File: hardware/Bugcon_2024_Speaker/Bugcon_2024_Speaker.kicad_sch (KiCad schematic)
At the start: 53 parts, among them J1 OLED, J2 Add_On, J4 Battery, J5 Battery, P1 USB_C_Plug_USB2.0, Q1 DMG3415U-7, SW1 ON, U1 ESP32-C6-WROOM-1U-N4, U2 XC6220B331MR-G

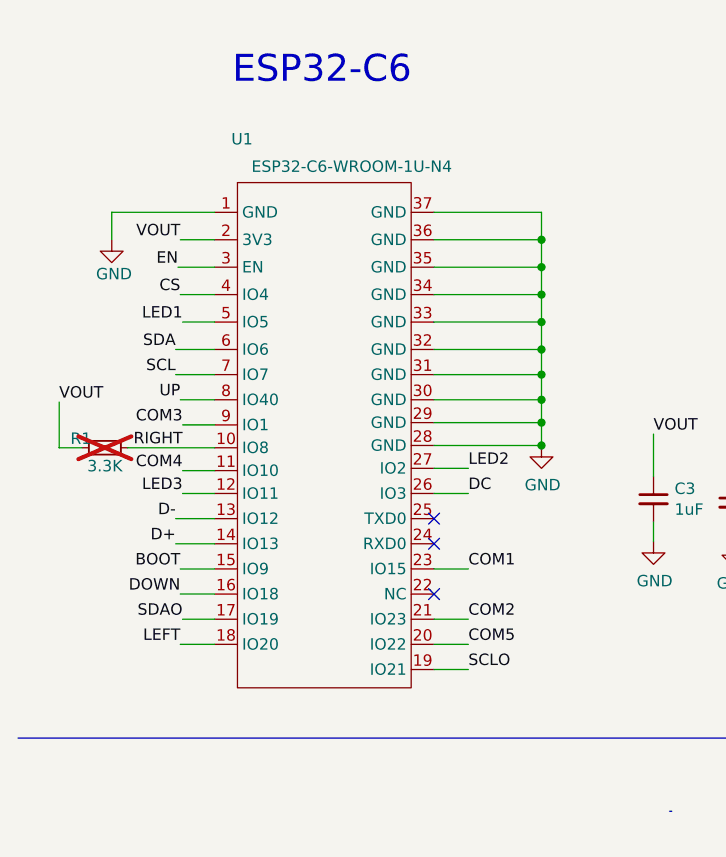
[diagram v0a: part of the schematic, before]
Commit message: feat(Hw):Update_Labels_And_route
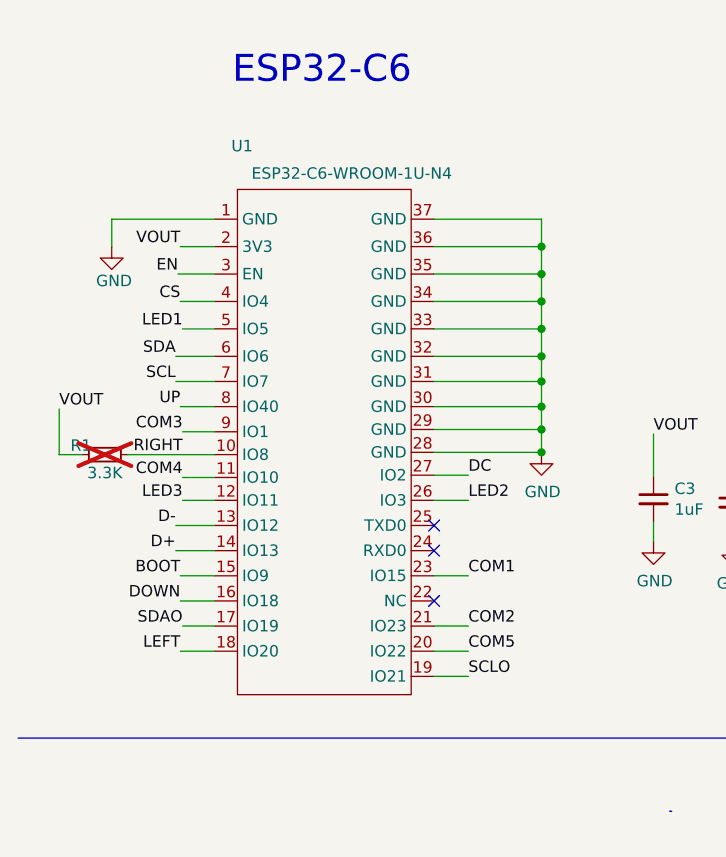
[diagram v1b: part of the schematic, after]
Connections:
- net DC: now also U1.27 (IO2); no longer U1.26 (IO3)
- net LED2: now also U1.26 (IO3); no longer U1.27 (IO2)
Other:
- moved on the sheet: R1, U1

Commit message: feat(Hw):Update_BOM
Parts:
- C1, C11, C12, C13, C14, C2, C3, C4, C5, C6, C7, D1, F1, J2, J4, J5, P1, Q1, R1, R2, R3, R4, R6, SW1, SW2, SW3, SW4, SW5, SW6, SW7, U2: Proveedor JLCPCB -> (none)
- D2, D3, D4, D5, D8: Proveedor (none) -> MOUSER
- J1: Proveedor (none) -> UNIT; manf# (none) -> GC9A01 Pantalla TFT LCD Circular 1.28 Pulgadas
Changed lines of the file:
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@@
 			)
 		)
-		(property "Proveedor" "JLCPCB"
+		(property "Proveedor" ""
 			(at 192.151 68.326 0)
 			(effects
@@
 			)
 		)
-		(property "Proveedor" "JLCPCB"
+		(property "Proveedor" ""
 			(at 193.294 55.118 0)
 			(effects
@@
 			)
 		)
-		(property "Proveedor" "JLCPCB"
+		(property "Proveedor" ""
 			(at 259.08 64.516 0)
 			(effects
@@
 			)
 		)
-		(property "Proveedor" "JLCPCB"
+		(property "Proveedor" ""
 			(at 193.294 52.578 0)
 			(effects
@@
 			)
 		)
-		(property "Proveedor" "JLCPCB"
+		(property "Proveedor" ""
 			(at 150.622 47.498 0)
 			(effects
@@
 			)
 		)
+		(property "Proveedor" "MOUSER"
+			(at 207.01 123.19 0)
+			(effects
+				(font
+					(size 1.27 1.27)
+				)
+				(hide yes)
+			)
+		)
 		(pin "3"
 		)
@@
 			)
 		)
-		(property "Proveedor" "JLCPCB"
+		(property "Proveedor" ""
 			(at 151.892 42.418 0)
 			(effects
@@
 			)
 		)
+		(property "Proveedor" "MOUSER"
+			(at 265.43 133.35 0)
+			(effects
+				(font
+					(size 1.27 1.27)
+				)
+				(hide yes)
+			)
+		)
 		(pin "3"
 		)
@@
 			)
 		)
-		(property "Proveedor" "JLCPCB"
+		(property "Proveedor" ""
 			(at 41.783 179.451 0)
 			(effects
@@
 			)
 		)
+		(property "Proveedor" "MOUSER"
+			(at 265.43 109.22 0)
+			(effects
+				(font
+					(size 1.27 1.27)
+				)
+				(hide yes)
+			)
+		)
 		(pin "3"
 		)
@@
 			)
 		)
-		(property "Proveedor" "JLCPCB"
+		(property "Proveedor" ""
 			(at 82.804 66.167 0)
 			(effects
@@
 			)
 		)
-		(property "Proveedor" "JLCPCB"
+		(property "Proveedor" ""
 			(at 259.08 48.006 0)
 			(effects
@@
 			)
 		)
-		(property "Proveedor" "JLCPCB"
+		(property "Proveedor" ""
 			(at 64.77 121.92 0)
 			(effects
@@
 			)
 		)
+		(property "Proveedor" "UNIT"
+			(at 143.51 121.92 0)
+			(effects
+				(font
+					(size 1.27 1.27)
+				)
+				(hide yes)
+			)
+		)
+		(property "manf#" "GC9A01 Pantalla TFT LCD Circular 1.28 Pulgadas"
+			(at 143.51 121.92 0)
+			(effects
+				(font
+					(size 1.27 1.27)
+				)
+				(hide yes)
+			)
+		)
 		(pin "3"
 		)
@@
 			)
 		)
-		(property "Proveedor" "JLCPCB"
+		(property "Proveedor" ""
 			(at 91.694 66.548 0)
 			(effects
@@
 			)
 		)
-		(property "Proveedor" "JLCPCB"
+		(property "Proveedor" ""
 			(at 146.304 180.848 0)
 			(effects
@@
 			)
 		)
-		(property "Proveedor" "JLCPCB"
+		(property "Proveedor" ""
 			(at 258.826 44.45 0)
 			(effects
@@
 			)
 		)
-		(property "Proveedor" "JLCPCB"
+		(property "Proveedor" ""
 			(at 100.584 66.548 0)
 			(effects
@@
 			)
 		)
-		(property "Proveedor" "JLCPCB"
+		(property "Proveedor" ""
 			(at 258.826 24.13 0)
 			(effects
@@
 			)
 		)
-		(property "Proveedor" "JLCPCB"
+		(property "Proveedor" ""
 			(at 131.064 57.658 0)
 			(effects
@@
 			)
 		)
-		(property "Proveedor" "JLCPCB"
+		(property "Proveedor" ""
 			(at 77.47 181.61 0)
 			(effects
@@
 			)
 		)
-		(property "Proveedor" "JLCPCB"
+		(property "Proveedor" ""
 			(at 21.844 61.214 0)
 			(effects
@@
 			)
 		)
-		(property "Proveedor" "JLCPCB"
+		(property "Proveedor" ""
 			(at 97.79 174.879 0)
 			(effects
@@
 			)
 		)
+		(property "Proveedor" "MOUSER"
+			(at 207.01 147.32 0)
+			(effects
+				(font
+					(size 1.27 1.27)
+				)
+				(hide yes)
+			)
+		)
 		(pin "3"
 		)
@@
 			)
 		)
-		(property "Proveedor" "JLCPCB"
+		(property "Proveedor" ""
 			(at 88.138 168.529 0)
 			(effects
@@
 			)
 		)
-		(property "Proveedor" "JLCPCB"
+		(property "Proveedor" ""
 			(at 56.515 177.419 0)
 			(effects
@@
 			)
 		)
-		(property "Proveedor" "JLCPCB"
+		(property "Proveedor" ""
 			(at 66.167 177.419 0)
 			(effects
@@
 			)
 		)
-		(property "Proveedor" "JLCPCB "
+		(property "Proveedor" ""
 			(at 184.404 47.498 0)
 			(effects
@@
 			)
 		)
-		(property "Proveedor" "JLCPCB"
+		(property "Proveedor" ""
 			(at 146.304 175.641 0)
 			(effects
@@
 			)
 		)
-		(property "Proveedor" "JLCPCB"
+		(property "Proveedor" ""
 			(at 192.024 70.358 0)
 			(effects
@@
 			)
 		)
-		(property "Proveedor" "JLCPCB"
+		(property "Proveedor" ""
 			(at 84.455 174.879 0)
 			(effects
@@
 			)
 		)
-		(property "Proveedor" "JLCPCB"
+		(property "Proveedor" ""
 			(at 257.556 80.01 0)
 			(effects
@@
 			)
 		)
+		(property "Proveedor" "MOUSER"
+			(at 265.43 157.48 0)
+			(effects
+				(font
+					(size 1.27 1.27)
+				)
+				(hide yes)
+			)
+		)
 		(pin "3"
 		)
@@
 			)
 		)
-		(property "Proveedor" "JLCPCB"
+		(property "Proveedor" ""
 			(at 259.08 27.686 0)
 			(effects
@@
 			)
 		)
-		(property "Proveedor" "JLCPCB"
+		(property "Proveedor" ""
 			(at 150.622 50.038 0)
 			(effects
@@
 			)
 		)
-		(property "Proveedor" "JLCPCB"
+		(property "Proveedor" ""
 			(at 257.81 83.566 0)
 			(effects
@@
 			)
 		)
-		(property "Proveedor" "JLCPCB"
+		(property "Proveedor" ""
 			(at 258.826 60.96 0)
 			(effects
